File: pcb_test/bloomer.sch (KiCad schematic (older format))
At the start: 202 parts, among them J1 USB_mini_micro_B, K1 KEYSW, K10 KEYSW, K11 KEYSW, K12 KEYSW, K13 KEYSW, K14 KEYSW, K15 KEYSW, K16 KEYSW, K17 KEYSW, K18 KEYSW, K19 KEYSW, K2 KEYSW, K20 KEYSW, K21 KEYSW, K22 KEYSW, K23 KEYSW, K24 KEYSW, K25 KEYSW, K26 KEYSW, K27 KEYSW, K28 KEYSW, K29 KEYSW, K3 KEYSW, K30 KEYSW, K31 KEYSW, K32 KEYSW, K33 KEYSW, K34 KEYSW, K35 KEYSW, K36 KEYSW, K37 KEYSW, K38 KEYSW, K39 KEYSW, K4 KEYSW, K40 KEYSW, K41 KEYSW, K42 KEYSW, K43 KEYSW, K44 KEYSW, K45 KEYSW, K46 KEYSW, K47 KEYSW, K48 KEYSW, K49 KEYSW, K5 KEYSW, K50 KEYSW, K51 KEYSW, K52 KEYSW, K53 KEYSW, K54 KEYSW, K55 KEYSW, K56 KEYSW, K57 KEYSW, K58 KEYSW, K59 KEYSW, K6 KEYSW, K60 KEYSW, K61 KEYSW, K62 KEYSW, K63 KEYSW, K64 KEYSW, K65 KEYSW, K66 KEYSW, K67 KEYSW, K68 KEYSW, K69 KEYSW, K7 KEYSW, K70 KEYSW, K71 KEYSW, K72 KEYSW, K73 KEYSW, K74 KEYSW, K75 KEYSW, K76 KEYSW, K77 KEYSW, K78 KEYSW, K79 KEYSW, K8 KEYSW, K80 KEYSW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

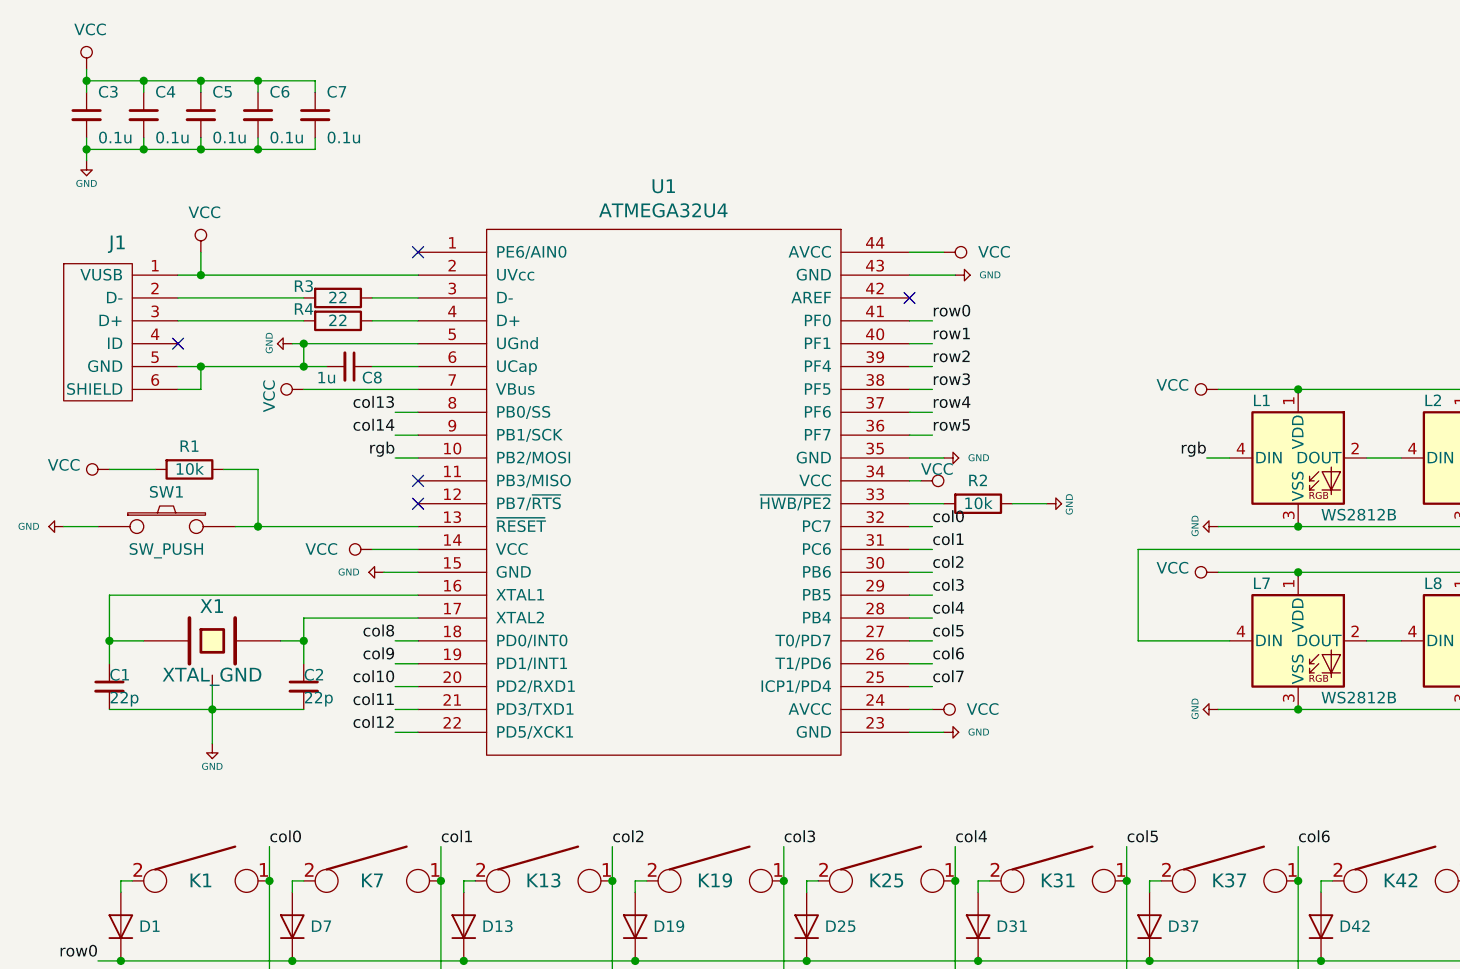
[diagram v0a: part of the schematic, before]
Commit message: Updates
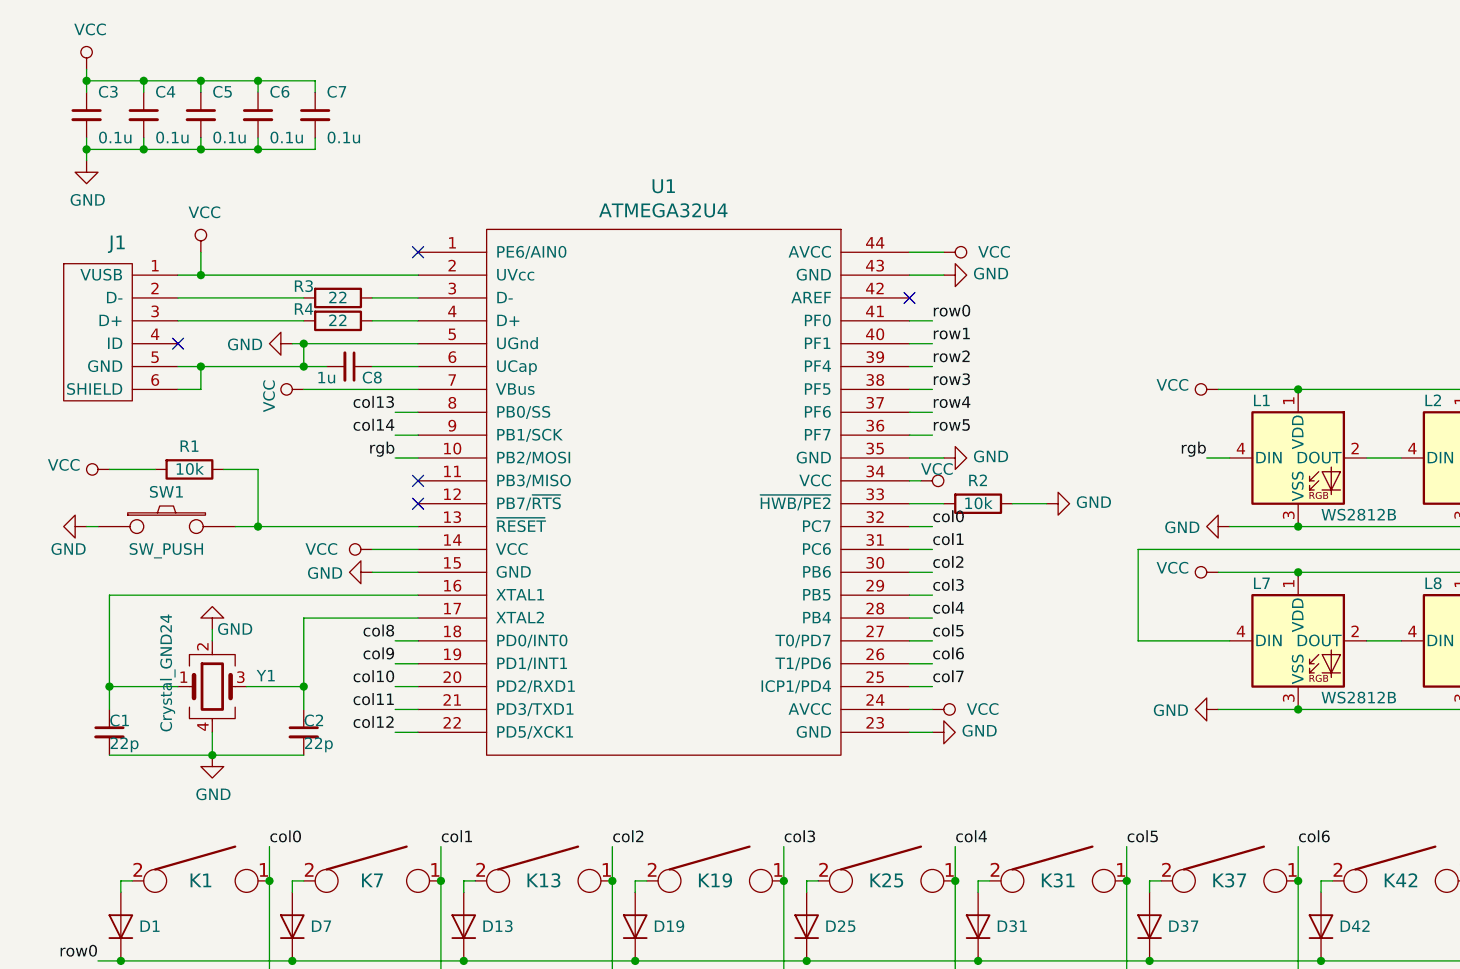
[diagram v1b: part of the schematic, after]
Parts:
- removed X1: XTAL_GND, Crystal:Crystal_SMD_TXC_7M-4Pin_3.2x2.5mm_HandSoldering, symbol keyboard_parts:XTAL_GND
- added Y1: Crystal_GND24, Crystal:Crystal_SMD_TXC_7M-4Pin_3.2x2.5mm_HandSoldering, symbol Device:Crystal_GND24
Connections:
- net at C1.1, U1.16 (XTAL1): now also Y1.1
- net at C2.1, U1.17 (XTAL2): now also Y1.3
- net +5V renamed GND
- net GND: now also Y1.2, Y1.4
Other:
- moved on the sheet: C1, C2
